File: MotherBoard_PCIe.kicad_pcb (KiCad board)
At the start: 2 copper layers, 90 x 196 mm, 40 parts, among them J1 Conn_01x02, J10 Bus_mechaken_PCIexpress_x16_1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, J11 Conn_01x03, J12 Conn_01x03, J2 Conn_01x02, J3 Conn_01x07, J4 Conn_01x07, J5 Bus_mechaken_PCIexpress_x16_1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, J6 Bus_mechaken_PCIexpress_x16_1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, J7 Bus_mechaken_PCIexpress_x16_1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, J8 Bus_mechaken_PCIexpress_x16_1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, J9 Bus_mechaken_PCIexpress_x16_1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, U1 L7812

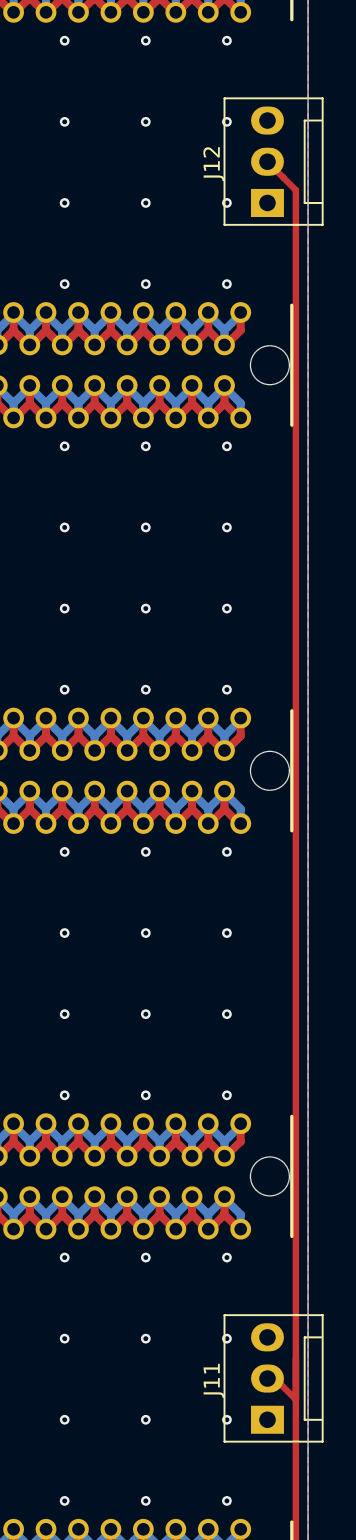
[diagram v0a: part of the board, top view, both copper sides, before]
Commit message: clean
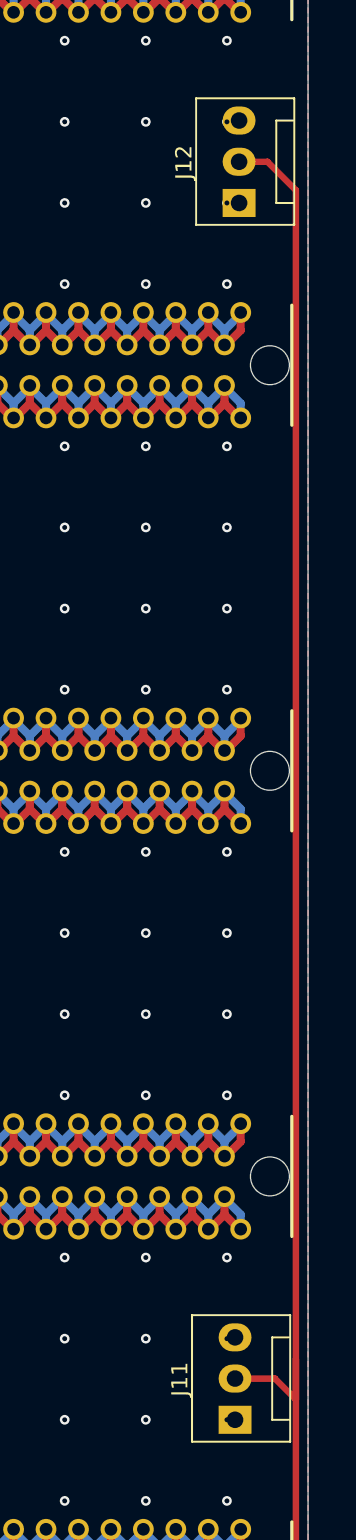
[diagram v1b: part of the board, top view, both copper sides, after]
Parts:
- moved J11 2.00 mm to (142.5, 153.5)
- moved J12 1.75 mm to (142.8, 78.5)
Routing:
- net +12V: track 190.4 -> 194.2 mm
- net Net-(J12-Pad3): vias 0 -> 1
- net Net-(J11-Pad3): vias 0 -> 1
- net GNDPWR: vias 250 -> 248
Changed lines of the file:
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@@
   )
   (setup
-    (last_trace_width 0.4)
+    (last_trace_width 0.25)
     (user_trace_width 0.2)
     (user_trace_width 0.4)
@@
   )
   (module Connector:FanPinHeader_1x03_P2.54mm_Vertical (layer F.Cu)
-    (at 144.5 78.5 90)
+    (at 142.75 78.5 90)
     (descr "3-pin CPU fan Through hole pin header, see http://www.formfactors.org/developer%5Cspecs%5Crev1_2_public.pdf")
     (tags "pin header 3-pin CPU fan")
@@
   )
   (module Connector:FanPinHeader_1x03_P2.54mm_Vertical (layer F.Cu)
-    (at 144.5 153.5 90)
+    (at 142.5 153.5 90)
     (descr "3-pin CPU fan Through hole pin header, see http://www.formfactors.org/developer%5Cspecs%5Crev1_2_public.pdf")
     (tags "pin header 3-pin CPU fan")
@@
   (via (at 142 83.5) (size 0.6) (drill 0.3) (layers F.Cu B.Cu) (net 2))
   (via (at 142 78.5) (size 0.6) (drill 0.3) (layers F.Cu B.Cu) (net 2))
-  (via (at 142 73.5) (size 0.6) (drill 0.3) (layers F.Cu B.Cu) (net 2))
+  (via (at 142 73.5) (size 0.6) (drill 0.3) (layers F.Cu B.Cu) (net 13))
   (via (at 142 68.5) (size 0.6) (drill 0.3) (layers F.Cu B.Cu) (net 2))
   (via (at 117 93.5) (size 0.6) (drill 0.3) (layers F.Cu B.Cu) (net 2))
@@
   (via (at 142 158.5) (size 0.6) (drill 0.3) (layers F.Cu B.Cu) (net 2))
   (via (at 142 153.5) (size 0.6) (drill 0.3) (layers F.Cu B.Cu) (net 2))
-  (via (at 142 148.5) (size 0.6) (drill 0.3) (layers F.Cu B.Cu) (net 2))
+  (via (at 142 148.5) (size 0.6) (drill 0.3) (layers F.Cu B.Cu) (net 11))
   (via (at 142 143.5) (size 0.6) (drill 0.3) (layers F.Cu B.Cu) (net 2))
   (via (at 117 168.5) (size 0.6) (drill 0.3) (layers F.Cu B.Cu) (net 2))
@@
   (segment (start 146 201) (end 146.25 200.75) (width 0.4) (layer F.Cu) (net 12))
   (segment (start 146.25 200.75) (end 146.25 149.75) (width 0.4) (layer F.Cu) (net 12))
-  (segment (start 145.5 76.96) (end 144.5 75.96) (width 0.4) (layer F.Cu) (net 12))
-  (segment (start 146.25 77.71) (end 145.5 76.96) (width 0.4) (layer F.Cu) (net 12))
-  (segment (start 146.25 152.25) (end 146.25 77.71) (width 0.4) (layer F.Cu) (net 12))
-  (segment (start 144.5 150.96) (end 144.96 150.96) (width 0.4) (layer F.Cu) (net 12))
   (segment (start 144.96 150.96) (end 146.25 152.25) (width 0.4) (layer F.Cu) (net 12))
+  (segment (start 142.5 150.96) (end 144.96 150.96) (width 0.4) (layer F.Cu) (net 12))
+  (segment (start 146.25 152.25) (end 146.25 77.71) (width 0.4) (layer F.Cu) (net 12))
+  (segment (start 146.25 77.71) (end 144.5 75.96) (width 0.4) (layer F.Cu) (net 12))
+  (segment (start 144.5 75.96) (end 142.75 75.96) (width 0.4) (layer F.Cu) (net 12))
   (zone (net 2) (net_name GNDPWR) (layer F.Cu) (hatch edge 0.508)
     (priority 5)
